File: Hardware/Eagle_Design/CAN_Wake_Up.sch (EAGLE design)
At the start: 32 parts, among them IC1 STM32F10XCXT6, IC4 LM1117MP-5.0, IC5 LM1117MP-3.3, Q1 8MHz

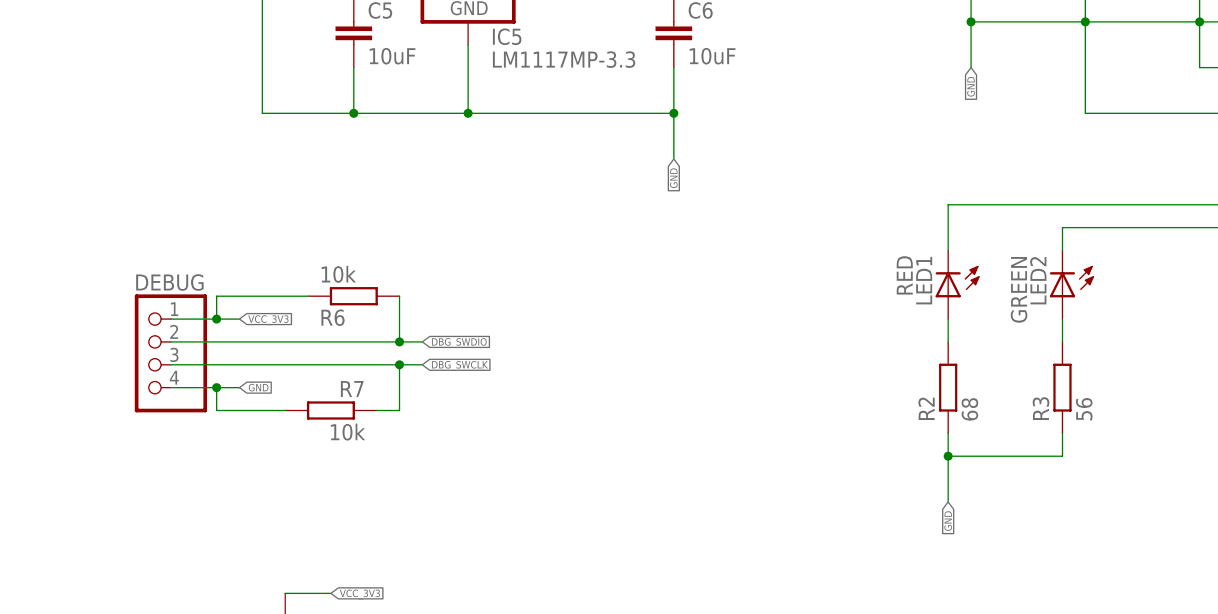
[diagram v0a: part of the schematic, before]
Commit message: Started on PCB layout.
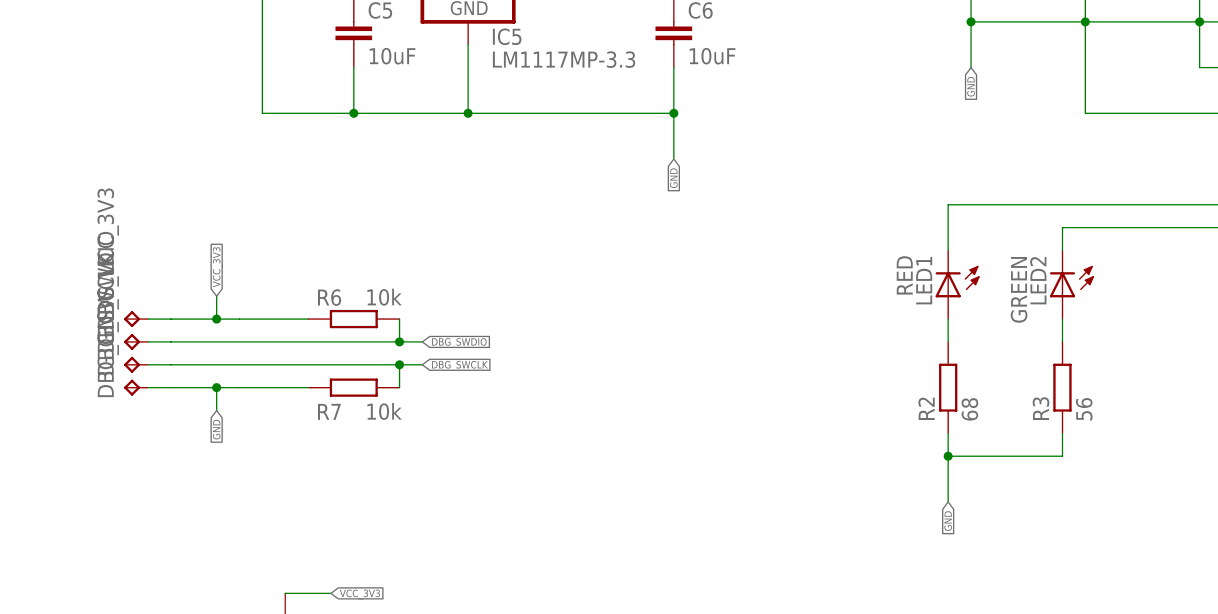
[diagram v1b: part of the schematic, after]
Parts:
- removed DEBUG: (no value), pinhead:PINHD-1X4
- added DBG_GND, DBG_SWCLK, DBG_SWDIO, DBG_VCC_3V3: TPB1,27, testpad:TPB1,27
- LED1, LED2: device led:LED3MM -> led:LEDSML0805
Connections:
- net DBG_SWCLK: now also DBG_SWCLK.TP; no longer DEBUG.3
- net DBG_SWDIO: now also DBG_SWDIO.TP; no longer DEBUG.2
- net GND: now also DBG_GND.TP; no longer DEBUG.4
- net VCC_3V3: now also DBG_VCC_3V3.TP; no longer DEBUG.1
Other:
- moved on the sheet: R6, R7
